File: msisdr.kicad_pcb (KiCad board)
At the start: 2 copper layers, 66 parts, among them J1 VCC_GPIO, J10 SMA_VHF1, J11 USB_OTG, J2 GPIO0, J3 GPIO1, J4 GPIO2, J5 GPIO3, J6 SMA_0_30MHZ, J7 SMA_30_60MHZ, J8 SMA_VHF2, J9 SMA_UHF, U1 msi2500, U2 msi001, U3 LP5900SDX-2.8, U4 AP7313-30SAG, Y1 24MHz

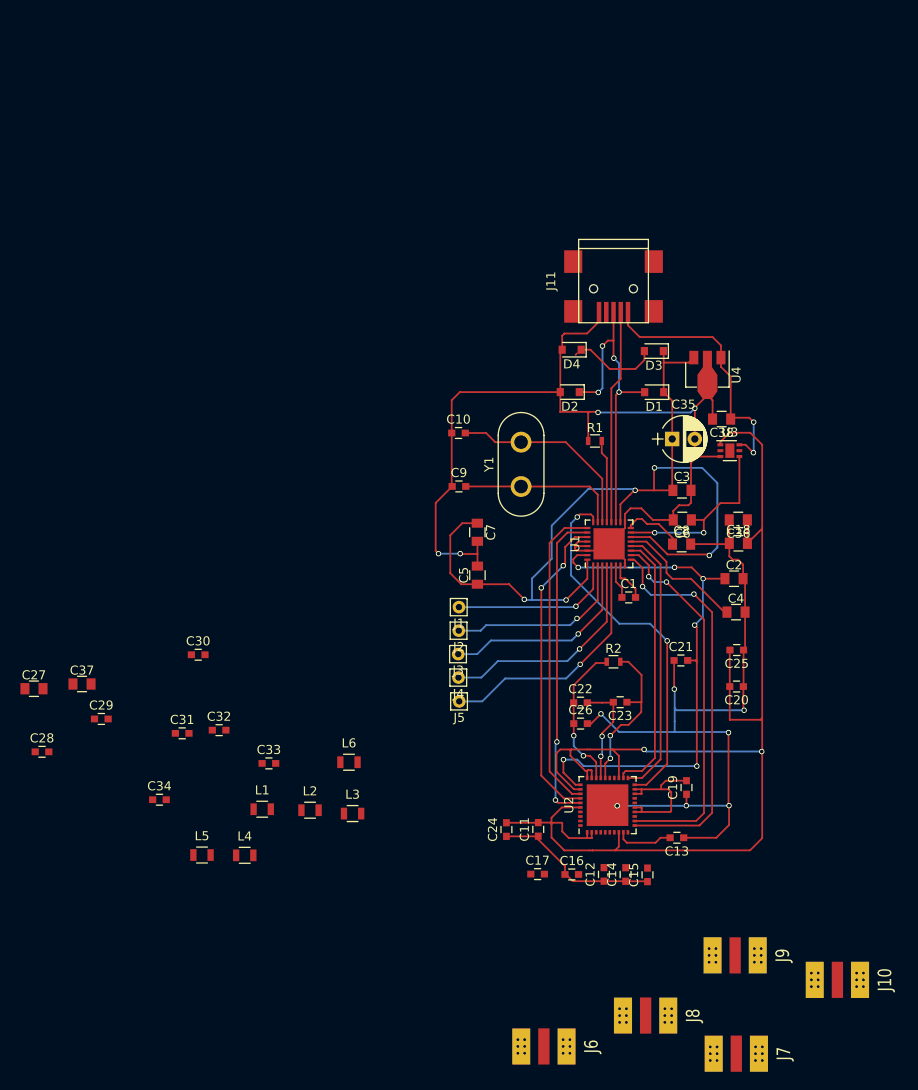
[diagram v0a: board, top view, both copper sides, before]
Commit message: finish pcb v1
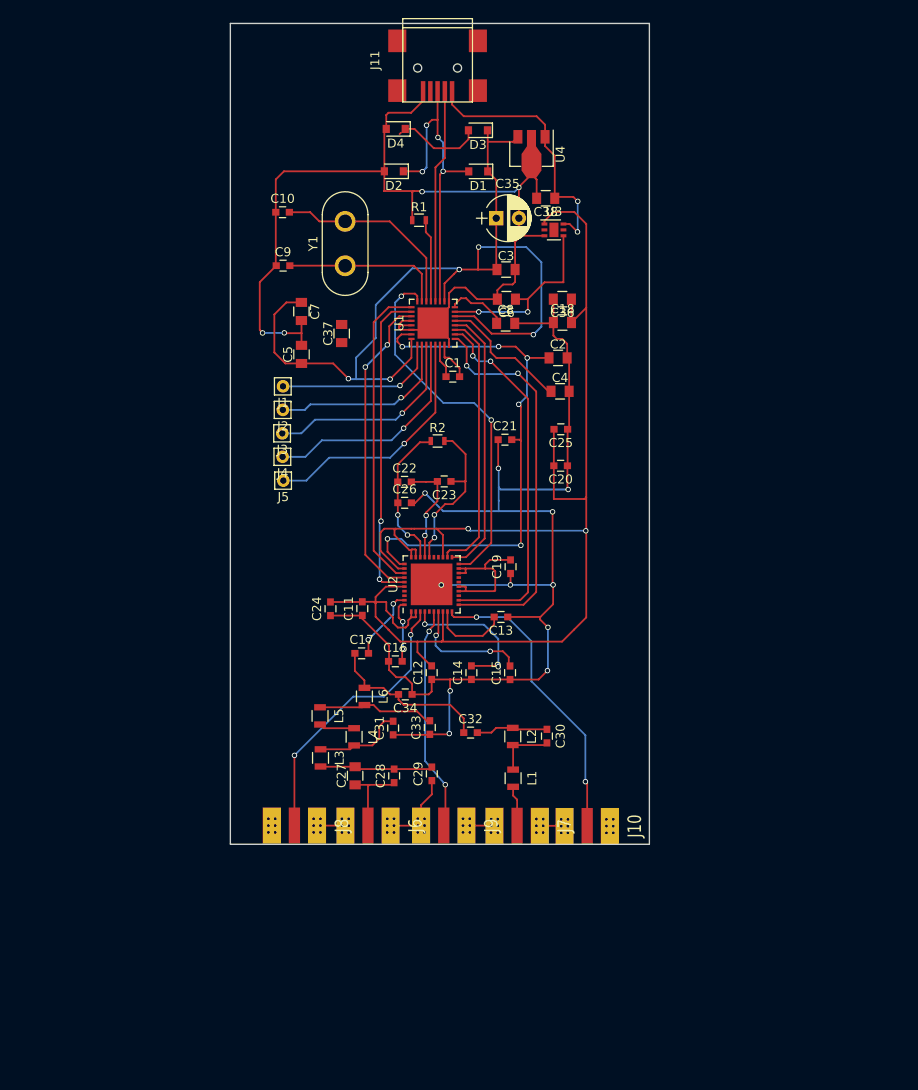
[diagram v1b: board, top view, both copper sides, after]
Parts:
- moved C37 48.2 mm to (125.4, 77.7), turned to 90 degrees
- moved J8 44.1 mm to (120.2, 134.6)
- moved C30 39.5 mm to (148.1, 122.2), turned to 270 degrees
- moved C28 39.0 mm to (131.2, 126.6), turned to 90 degrees
- moved C29 37.0 mm to (135.4, 126.4), turned to 90 degrees
- moved C27 36.8 mm to (126.9, 126.6), turned to 90 degrees
- moved J9 35.2 mm to (136.7, 134.6)
- moved J7 34.9 mm to (144.8, 134.6)
- moved J10 32.4 mm to (152.5, 134.6)
- moved C17 31.2 mm to (127.6, 113.0)
- moved D4 31.2 mm to (131.4, 55.1)
- moved C10 31.2 mm to (118.9, 64.3)
- moved C11 31.2 mm to (127.7, 108.1)
- moved C18 31.2 mm to (149.8, 76.5)
- moved C22 31.2 mm to (132.4, 94.1)
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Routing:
- net GND: track 216.4 -> 266.4 mm, vias 11 -> 15
- net VHF_50_120MHZ: track 0.00 -> 33.3 mm, vias 0 -> 2
- net VHF_120_250MHZ: track 0.00 -> 31.4 mm, vias 0 -> 2
- net UHF_400_1000MHZ: track 0.00 -> 24.9 mm, vias 0 -> 2
- net HFPORT: track 0.00 -> 18.5 mm
- net Net-(C14-Pad2): track 0.00 -> 16.3 mm, vias 0 -> 2
- net Net-(C15-Pad2): track 0.00 -> 13.5 mm, vias 0 -> 2
- net Net-(C33-Pad2): track 0.00 -> 12.9 mm
- net Net-(C27-Pad2): track 0.00 -> 12.5 mm
- net Net-(C31-Pad2): track 0.00 -> 10.1 mm
- net Net-(C27-Pad1): track 0.00 -> 8.98 mm
- net Net-(C17-Pad2): track 0.00 -> 8.02 mm, vias 0 -> 2
- net Net-(C30-Pad1): track 0.00 -> 7.97 mm
- net VRF: track 147.5 -> 154.8 mm
- net Net-(C16-Pad2): track 0.00 -> 6.97 mm, vias 0 -> 2
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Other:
- board outline added: 46.3 x 90.7 mm
